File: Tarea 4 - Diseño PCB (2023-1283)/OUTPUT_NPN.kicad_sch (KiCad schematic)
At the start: 8 parts

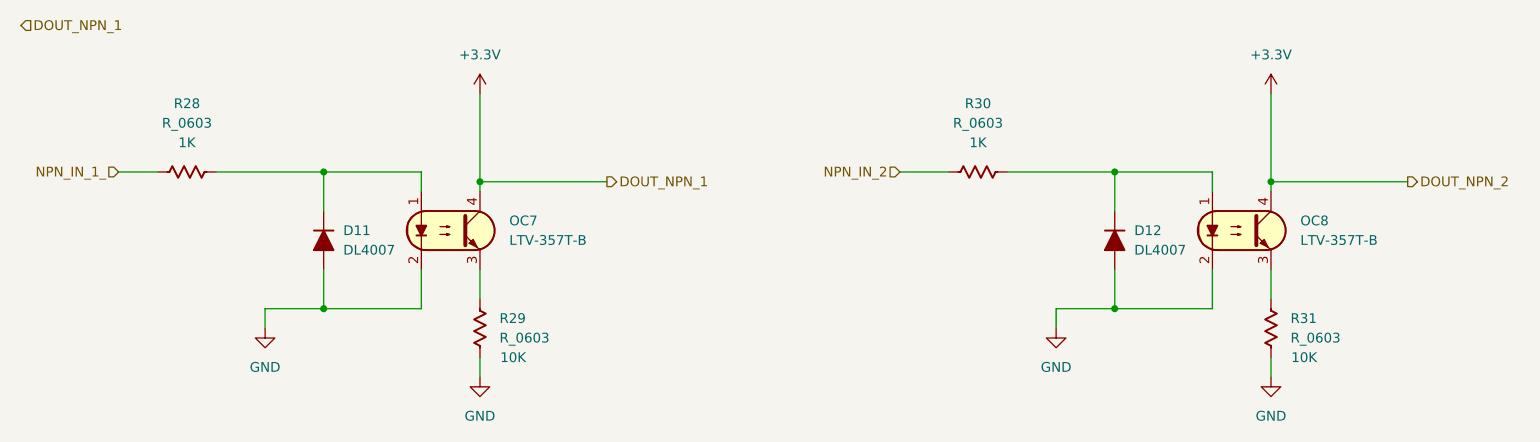
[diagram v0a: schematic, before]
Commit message: Complete
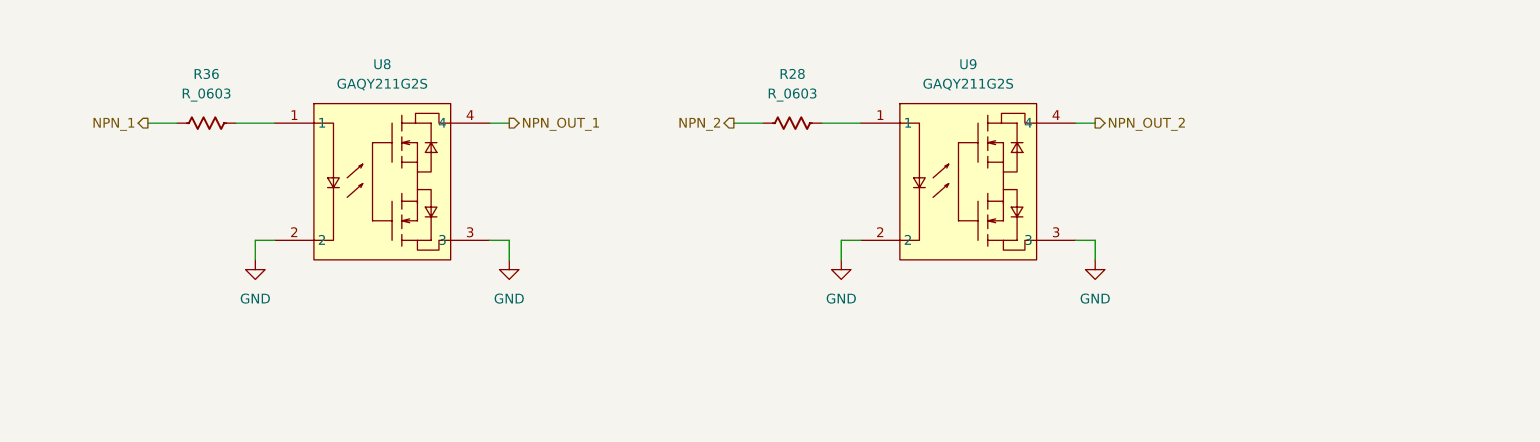
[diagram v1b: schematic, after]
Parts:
- removed D11, D12: DL4007, PCM_Diode_SMD_AKL:D_MELF, symbol PCM_Diode_AKL:DL4007
- removed OC7, OC8: LTV-357T-B, PCM_Package_SO_AKL:SO-4_4.4x3.9mm_P2.54mm, symbol PCM_Optocoupler_AKL:LTV-357T-B
- removed R29, R30, R31: R_0603, PCM_Resistor_SMD_AKL:R_0603_1608Metric, symbol PCM_Resistor_US_AKL:R_0603
- added R36: R_0603, PCM_Resistor_SMD_AKL:R_0603_1608Metric, symbol PCM_Resistor_US_AKL:R_0603
- added U8, U9: GAQY211G2S, Battery:GQRLY, symbol RLY:GAQY211G2S
- R28: Field5 1K -> (none)
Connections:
- net GND: now also U8.2, U8.3, U9.2, U9.3
- net at R28.1: now also U9.1
- net NPN_IN_1_ renamed NPN_2
- new net: R36.1, U8.1
- new net NPN_1: R36.2
- new net NPN_OUT_1: U8.4
- new net NPN_OUT_2: U9.4
